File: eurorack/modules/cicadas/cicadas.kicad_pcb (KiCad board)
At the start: 2 copper layers, 42.6 x 128.5 mm, 79 parts, among them J1 Conn_02x05_Odd_Even, J10 AudioJack2_SwitchT, J11 AudioJack2_SwitchT, J2 AVR-ISP-6, J3 AudioJack2_SwitchT, J4 AudioJack2_SwitchT, J5 AudioJack2_SwitchT, J6 AudioJack2_SwitchT, J7 AudioJack2_SwitchT, J8 AudioJack2_SwitchT, J9 AudioJack2_SwitchT, U1 L78L33_SOT89, U2 ATmega328P-A, U3 MCP4822, U4 MCP4822

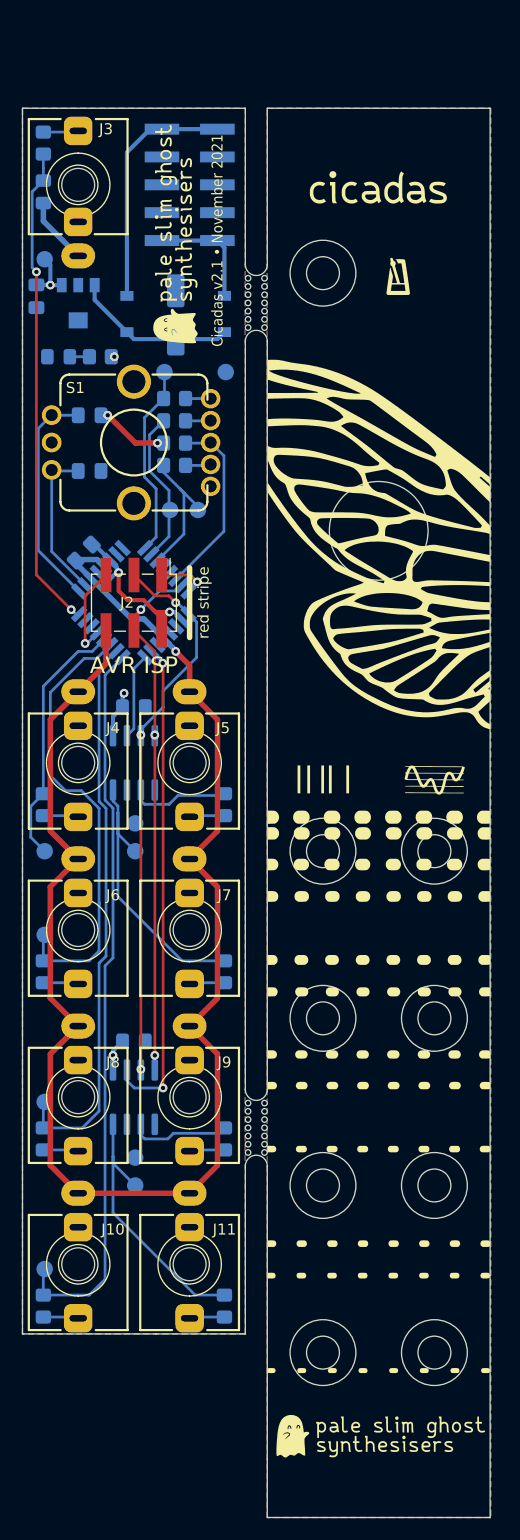
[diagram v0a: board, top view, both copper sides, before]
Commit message: initial work on cicadas v3
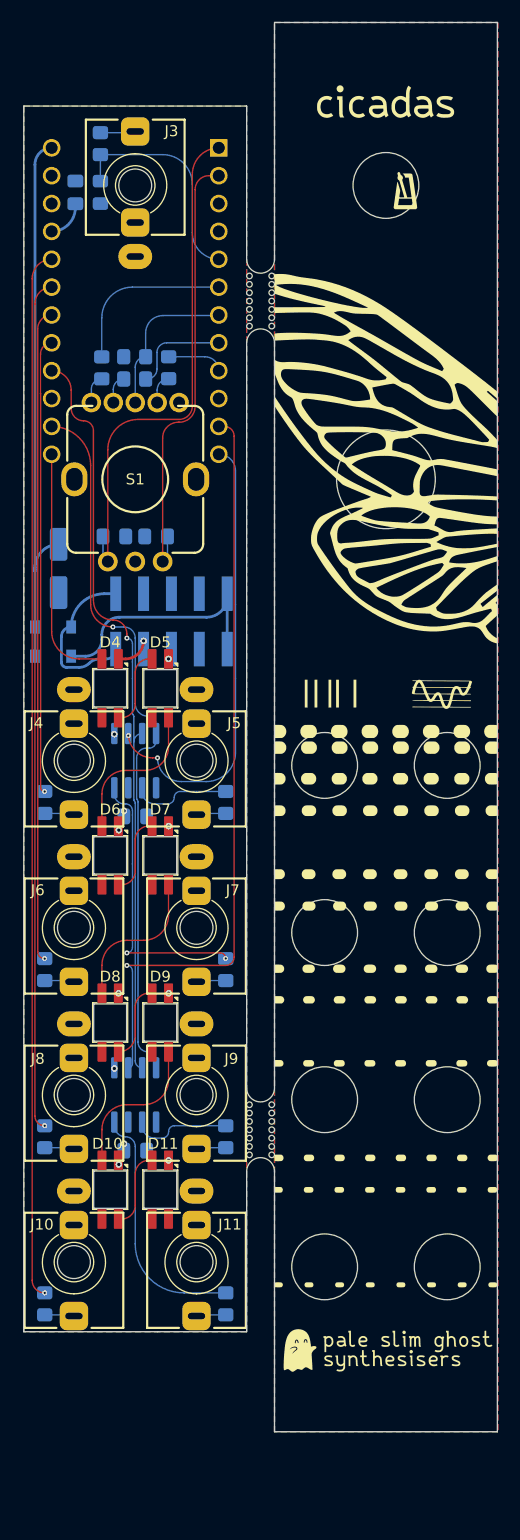
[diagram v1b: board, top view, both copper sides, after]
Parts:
- removed ? (x21): , 
- removed C2: 100n, Capacitor_SMD:C_0805_2012Metric_Pad1.18x1.45mm_HandSolder
- removed J2: AVR-ISP-6, Connector_PinHeader_2.54mm:PinHeader_2x03_P2.54mm_Vertical_SMD
- removed R2: R, Resistor_SMD:R_0805_2012Metric_Pad1.20x1.40mm_HandSolder
- removed TP1: 3.3V, TestPoint:TestPoint_Pad_D1.5mm
- removed TP10: B, TestPoint:TestPoint_Pad_D1.5mm
- removed TP11: A4, TestPoint:TestPoint_Pad_D1.5mm
- removed TP12: A3, TestPoint:TestPoint_Pad_D1.5mm
- removed TP13: GND, TestPoint:TestPoint_Pad_D1.5mm
- removed TP2: D4, TestPoint:TestPoint_Pad_D1.5mm
- removed TP3: D3, TestPoint:TestPoint_Pad_D1.5mm
- removed TP4: D2, TestPoint:TestPoint_Pad_D1.5mm
- removed TP5: A2, TestPoint:TestPoint_Pad_D1.5mm
- removed TP6: D1, TestPoint:TestPoint_Pad_D1.5mm
- removed TP7: A1, TestPoint:TestPoint_Pad_D1.5mm
- removed TP8: R, TestPoint:TestPoint_Pad_D1.5mm
- removed TP9: G, TestPoint:TestPoint_Pad_D1.5mm
- removed U2: ATmega328P-A, Package_QFP:TQFP-32_7x7mm_P0.8mm
- removed mouse-bite-2.54mm-slot: VAL**, Pale Slim Ghost:mousebite-2x5mm
- removed the mouse-bite-2mm-slot at (72.0, 68.8)
- added D10: SK6812MINI, Pale Slim Ghost:SK6812MINI-E, F.Cu at (58.7, 149.6)
- added D11: SK6812MINI, Pale Slim Ghost:SK6812MINI-E, F.Cu at (63.2, 149.6)
- added D5: SK6812MINI, Pale Slim Ghost:SK6812MINI-E, F.Cu at (63.2, 103.9)
- added D6: SK6812MINI, Pale Slim Ghost:SK6812MINI-E, F.Cu at (58.7, 119.1)
- added D7: SK6812MINI, Pale Slim Ghost:SK6812MINI-E, F.Cu at (63.2, 119.1)
- added D8: SK6812MINI, Pale Slim Ghost:SK6812MINI-E, F.Cu at (58.7, 134.4)
- added D9: SK6812MINI, Pale Slim Ghost:SK6812MINI-E, F.Cu at (63.2, 134.4)
- added H1: MountingHole, Pale Slim Ghost:eurorack panel mounting slot, F.Cu at (81.2, 46.2)
- added H10: MountingHole, Pale Slim Ghost:hole 6mm (jack panel), F.Cu at (78.2, 156.6)
- added H11: MountingHole, Pale Slim Ghost:hole 6mm (jack panel), F.Cu at (89.4, 156.6)
- added H12: MountingHole, Pale Slim Ghost:eurorack panel mounting slot, F.Cu at (81.2, 168.7)
- added H2: MountingHole, Pale Slim Ghost:hole 6mm (jack panel), F.Cu at (83.8, 58.0)
- added H3: MountingHole, Pale Slim Ghost:hole 9mm (encoder panel), F.Cu at (83.8, 84.8)
- added H4: MountingHole, Pale Slim Ghost:hole 6mm (jack panel), F.Cu at (78.2, 110.9)
- added H5: MountingHole, Pale Slim Ghost:hole 6mm (jack panel), F.Cu at (89.4, 110.9)
- added H6: MountingHole, Pale Slim Ghost:hole 6mm (jack panel), F.Cu at (78.2, 126.2)
- added H7: MountingHole, Pale Slim Ghost:hole 6mm (jack panel), F.Cu at (89.4, 126.2)
- added H8: MountingHole, Pale Slim Ghost:hole 6mm (jack panel), F.Cu at (78.2, 141.4)
- added H9: MountingHole, Pale Slim Ghost:hole 6mm (jack panel), F.Cu at (89.4, 141.4)
- added mouse-bite-2mm-slot: VAL**, Pale Slim Ghost:mousebite-2.54x5.08mm, F.Cu at (72.4, 144.1)
- added mouse-bite-2mm-slot: VAL**, Pale Slim Ghost:mousebite-2.54x5.08mm, F.Cu at (72.4, 68.6)
- D3: footprint LED_SMD:LED_0805_2012Metric_Pad1.15x1.40mm_HandSolder -> Diode_SMD:D_0805_2012Metric_Pad1.15x1.40mm_HandSolder
- D4: value LED -> SK6812MINI; footprint LED_SMD:LED_0805_2012Metric_Pad1.15x1.40mm_HandSolder -> Pale Slim Ghost:SK6812MINI-E; moved to F.Cu
- G***: moved to B.Cu
- J10, J11, J3, J4, J5, J6, J7, J8, J9: footprint AudioJacks:Jack_3.5mm_QingPu_WQP-PJ398SM_Vertical -> Pale Slim Ghost:Jack_3.5mm_QingPu_WQP-PJ398SM_Vertical
- U1: value L78L33_SOT89 -> ProMicro; footprint Package_TO_SOT_SMD:SOT-89-3 -> promicro:ProMicro-NoSilk
- moved G*** 64.8 mm to (60.7, 127.1), turned to 180 degrees
- moved J1 39.8 mm to (64.3, 97.8), turned to 90 degrees
- moved C4 32.8 mm to (55.5, 58.7), turned to 90 degrees
- moved D2 32.5 mm to (53.5, 98.3), turned to 0 degrees
- moved D1 31.9 mm to (53.5, 101.0), turned to 0 degrees
- moved D4 30.6 mm to (58.7, 103.9), turned to 90 degrees
- moved C1 25.5 mm to (54.0, 93.0), turned to -90 degrees
- moved C3 11.3 mm to (59.1, 90.0)
- moved C6 9.96 mm to (61.0, 146.1)
- moved C7 9.96 mm to (61.0, 115.6)
- moved R5 8.92 mm to (64.0, 74.7), turned to 90 degrees
- moved R8 8.67 mm to (60.9, 73.7)
- moved C5 8.51 mm to (62.9, 90.0), turned to 180 degrees
- moved G*** 7.85 mm to (83.8, 107.7)
- moved R3 7.20 mm to (57.9, 74.7), turned to 90 degrees
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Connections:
- D4 pad 1: GND -> +3V3
- U1 pad 1: +3V3 -> encoder A
- U1 pad 2: GND -> encoder B
- U1 pad 3: +12V -> GND
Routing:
- net GND: track 153.0 -> 5.81 mm, vias 3 -> 8
- net +12V: track 14.9 -> 51.0 mm
- net CS1: track 7.83 -> 41.4 mm, vias 0 -> 2
- net D4: track 66.6 -> 95.8 mm, vias 0 -> 1
- net encoder A: track 20.6 -> 47.4 mm
- net encoder B: track 14.3 -> 40.9 mm
- net D3: track 51.3 -> 77.8 mm, vias 0 -> 1
- net CS2: track 44.8 -> 69.4 mm, vias 2 -> 1
- net +3V3: track 28.9 -> 4.95 mm, vias 6 -> 4
- net clock in: track 44.3 -> 20.4 mm, vias 2 -> 0
- net LED: track 0.00 -> 22.1 mm
- net SCK: track 50.4 -> 69.0 mm, vias 3 -> 1
- net COPI: track 47.7 -> 66.2 mm, vias 3 -> 1
- net D1: track 23.4 -> 41.7 mm, vias 0 -> 1
- net D2: track 41.7 -> 59.7 mm, vias 0 -> 1
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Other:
- board size 42.6 x 128.5 mm -> 43.2 x 128.5 mm
- board text added: "Cicadas v3 April 2022"
- board text added: "either way ↓"
- board text removed: "AVR ISP"
- board text removed: "Cicadas v2.1 • November 2021"
- board text removed: "red stripe"
- board text removed: "← either way →"
